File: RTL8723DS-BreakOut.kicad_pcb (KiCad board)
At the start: 2 copper layers, 50 x 40 mm, 25 parts, among them J1 PWR_TER, J2 PWR_CONN, J3 WL_ACT_CONN, J4 BT_ACT_CONN, J5 CLK_CONN, J6 INT_SIG_CONN, J7 BT_CONN, J8 WL_CONN

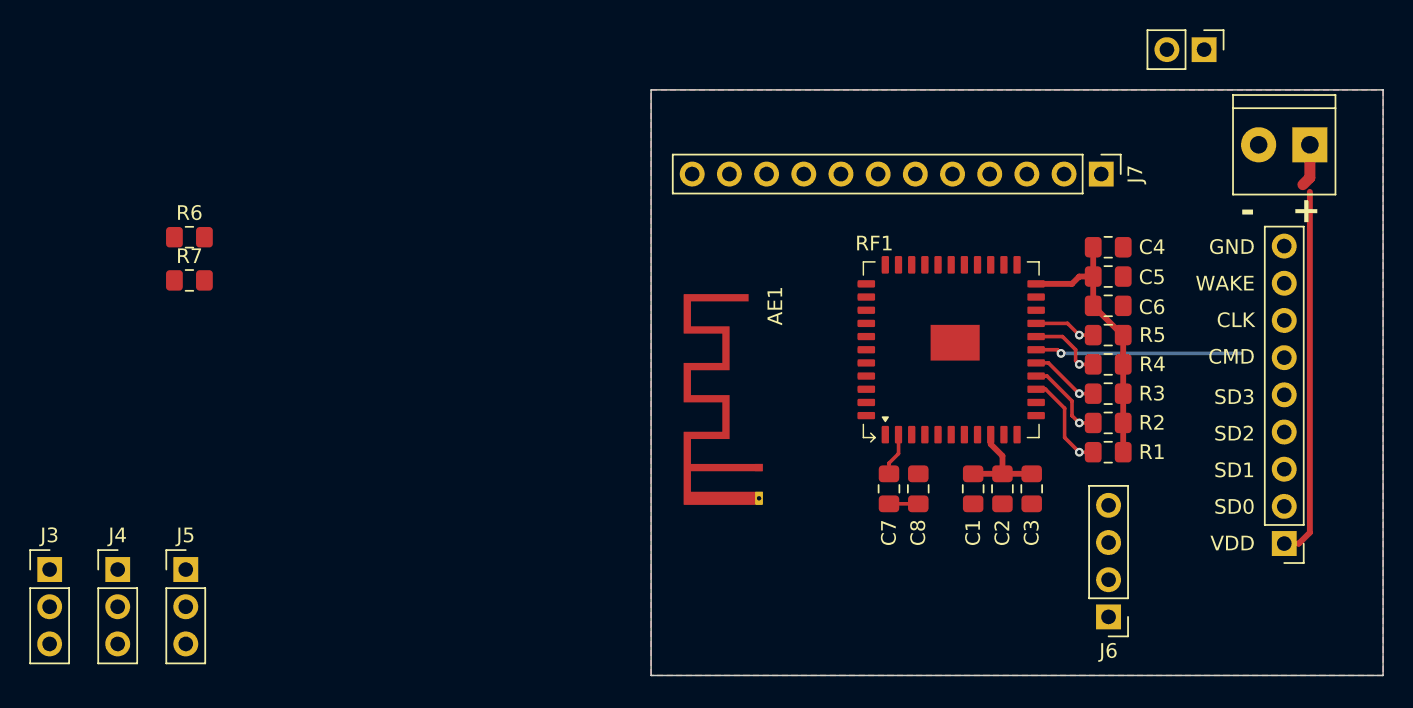
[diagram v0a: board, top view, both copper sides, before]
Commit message: Update design
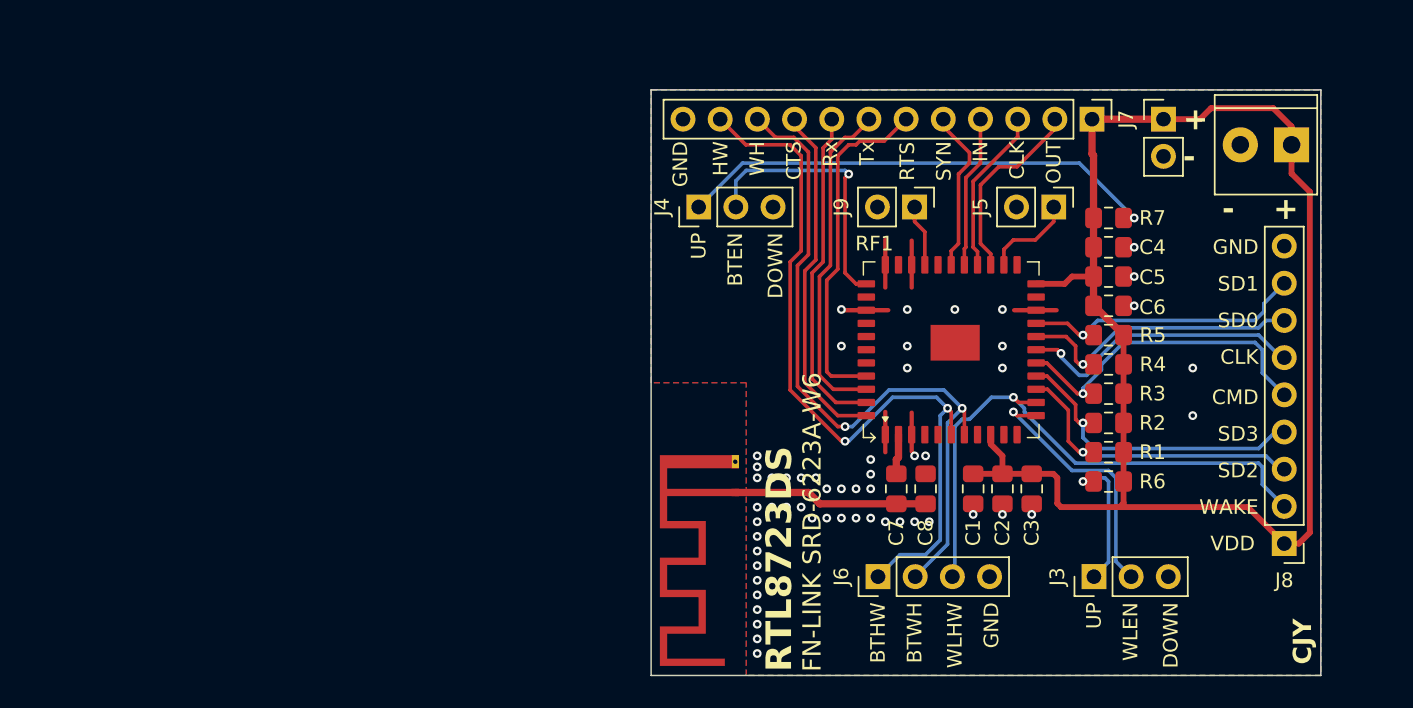
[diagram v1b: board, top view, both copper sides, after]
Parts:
- added J9: XTAL_CONN, Connector_PinHeader_2.54mm:PinHeader_1x02_P2.54mm_Vertical, F.Cu at (168.0, 73.0)
- AE1: footprint RF_Antenna:Texas_SWRA117D_2.4GHz_Right -> RF_Antenna:Texas_SWRA117D_2.4GHz_Left
- J5: value CLK_CONN -> SUSCLK_CONN; footprint Connector_PinHeader_2.54mm:PinHeader_1x03_P2.54mm_Vertical -> Connector_PinHeader_2.54mm:PinHeader_1x02_P2.54mm_Vertical
- moved J3 71.3 mm to (180.2, 98.2), turned to 90 degrees
- moved R6 65.0 mm to (181.2, 91.8), turned to 180 degrees
- moved J5 64.2 mm to (177.5, 73.0), turned to -90 degrees
- moved R7 62.9 mm to (181.2, 73.8)
- moved J4 46.8 mm to (153.2, 73.0), turned to 90 degrees
- moved J6 16.0 mm to (165.5, 98.2), turned to 90 degrees
- moved J2 5.50 mm to (185.0, 67.0), turned to 0 degrees
- moved J7 3.80 mm to (180.1, 67.0)
- moved AE1 2.35 mm to (155.8, 92.5)
- moved J1 1.25 mm to (192.0, 68.8)
- moved C7 0.50 mm to (166.8, 92.2)
- moved C8 0.50 mm to (168.8, 92.2)
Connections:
- J5 pad 2: MAIN_XTAL_IN -> GND
- J7 pad 10: HOST_WAKE_BT -> BT_WAKE_HOST
- J7 pad 11: BT_WAKE_HOST -> HOST_WAKE_BT
- J8 pad 2: SD_D0 -> WL_HOST_WAKE
- J8 pad 3: SD_D1 -> SD_D2
- J8 pad 4: SD_D2 -> SD_D3
- J8 pad 5: SD_D3 -> SD_CMD
- J8 pad 6: SD_CMD -> SD_CLK
- J8 pad 7: SD_CLK -> SD_D0
- J8 pad 8: WL_HOST_WAKE -> SD_D1
- RF1 pad 1: (no net) -> GND
- RF1 pad 20: (no net) -> GND
- RF1 pad 3: (no net) -> GND
- RF1 pad 31: (no net) -> GND
- RF1 pad 33: (no net) -> GND
- RF1 pad 36: (no net) -> GND
- RF1 pad 45: (no net) -> GND
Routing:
- net HOST_WAKE_BT: track 0.00 -> 53.0 mm, vias 0 -> 2
- net VBAT: track 54.2 -> 103.7 mm
- net BT_WAKE_HOST: track 0.00 -> 49.4 mm, vias 0 -> 2
- net WL_HOST_WAKE: track 0.00 -> 39.3 mm, vias 0 -> 1
- net Net-(J4-Pin_1): track 0.00 -> 33.3 mm, vias 0 -> 1
- net UART_CTS: track 0.00 -> 24.0 mm
- net UART_RTS: track 0.00 -> 23.6 mm
- net UART_OUT: track 0.00 -> 22.8 mm
- net UART_IN: track 0.00 -> 22.7 mm
- net BT_DIS: track 0.00 -> 18.5 mm, vias 0 -> 1
- net SD_CMD: track 4.77 -> 22.8 mm
- net GND: track 0.00 -> 18.0 mm, vias 0 -> 55
- net WL_DIS: track 0.00 -> 17.7 mm, vias 0 -> 1
- net SD_D1: track 4.23 -> 19.8 mm
- net SD_D3: track 5.81 -> 21.4 mm
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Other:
- board size 50 x 40 mm -> 45.8 x 40 mm
- board text added: "BTEN"
- board text added: "BTHW"
- board text added: "BTWH"
- board text added: "CJY"
- board text added: "CTS"
- board text added: "DOWN"
- board text added: "FN-LINK SRD-6223A-W6"
- board text added: "HW"
- board text added: "IN"
- board text added: "OUT"
- board text added: "RTL8723DS"
- board text added: "RTS"
- board text added: "Rx"
- board text added: "SYN"
- board text added: "Tx"
- board text added: "UP"
- board text added: "WH"
- board text added: "WLEN"
- board text added: "WLHW"
